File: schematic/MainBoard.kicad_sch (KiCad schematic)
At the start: 0 parts

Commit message: Progress on KiCAD schematics
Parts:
- added U1: LPC1115FBD48-303, Package_QFP:LQFP-48_7x7mm_P0.5mm, symbol MCU_NXP_LPC:LPC1115FBD48-303
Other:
- title: (none) -> Da Vinci Jr. 1.0 Main Board schematic
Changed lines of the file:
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@@
 	(generator_version "10.0")
 	(paper "A4")
+	(title_block
+		(title "Da Vinci Jr. 1.0 Main Board schematic")
+		(date "2026-08-26")
+		(rev "1")
+	)
+	(symbol
+		(lib_id "MCU_NXP_LPC:LPC1115FBD48-303")
+		(at 224.79 73.66 0)
+		(unit 1)
+		(body_style 1)
+		(exclude_from_sim no)
+		(in_bom yes)
+		(on_board yes)
+		(in_pos_files yes)
+		(dnp no)
+		(fields_autoplaced yes)
+		(property "Reference" "U1"
+			(at 229.4733 34.29 0)
+			(show_name no)
+			(do_not_autoplace no)
+			(effects
+				(font
+					(size 1.27 1.27)
+				)
+				(justify left)
+			)
+		)
+		(property "Value" "LPC1115FBD48-303"
+			(at 229.4733 36.83 0)
+			(show_name no)
+			(do_not_autoplace no)
+			(effects
+				(font
+					(size 1.27 1.27)
+				)
+				(justify left)
+			)
+		)
+		(property "Footprint" "Package_QFP:LQFP-48_7x7mm_P0.5mm"
+			(at 247.65 35.56 0)
+			(hide yes)
+			(show_name no)
+			(do_not_autoplace no)
+			(effects
+				(font
+					(size 1.27 1.27)
+				)
+			)
+		)
+		(property "Datasheet" "http://www.nxp.com/docs/en/data-sheet/LPC111X.pdf"
+			(at 273.05 58.42 0)
+			(hide yes)
+			(show_name no)
+			(do_not_autoplace no)
+			(effects
+				(font
+					(size 1.27 1.27)
+				)
+			)
+		)
+		(property "Description" "32-bit ARM Cortex-M0 microcontroller, 64KB flash, 8KB SRAM, power profile"
+			(at 224.79 73.66 0)
+			(hide yes)
+			(show_name no)
+			(do_not_autoplace no)
+			(effects
+				(font
+					(size 1.27 1.27)
+				)
+			)
+		)
+		(pin "14"
+		)
+		(pin "8"
+		)
+		(pin "7"
+		)
+		(pin "9"
+		)
+		(pin "6"
+		)
+		(pin "5"
+		)
+		(pin "13"
+		)
+		(pin "4"
+		)
+		(pin "12"
+		)
+		(pin "11"
+		)
+		(pin "10"
+		)
+		(pin "3"
+		)
+		(pin "17"
+		)
+		(pin "16"
+		)
+		(pin "24"
+		)
+		(pin "25"
+		)
+		(pin "15"
+		)
+		(pin "20"
+		)
+		(pin "26"
+		)
+		(pin "19"
+		)
+		(pin "22"
+		)
+		(pin "18"
+		)
+		(pin "23"
+		)
+		(pin "21"
+		)
+		(pin "2"
+		)
+		(pin "36"
+		)
+		(pin "35"
+		)
+		(pin "34"
+		)
+		(pin "33"
+		)
+		(pin "32"
+		)
+		(pin "31"
+		)
+		(pin "30"
+		)
+		(pin "29"
+		)
+		(pin "28"
+		)
+		(pin "27"
+		)
+		(pin "47"
+		)
+		(pin "46"
+		)
+		(pin "45"
+		)
+		(pin "44"
+		)
+		(pin "43"
+		)
+		(pin "42"
+		)
+		(pin "41"
+		)
+		(pin "48"
+		)
+		(pin "40"
+		)
+		(pin "38"
+		)
+		(pin "39"
+		)
+		(pin "37"
+		)
+		(pin "1"
+		)
+		(instances
+			(project "DaVinciJr1.0"
+				(path "/1e12c736-bef9-40e8-b505-1000ff77a2bb/d610c2e8-63cd-4e0f-98e2-bf1a99df609b"
+					(reference "U1")
+					(unit 1)
+				)
+			)
+		)
+	)
 )

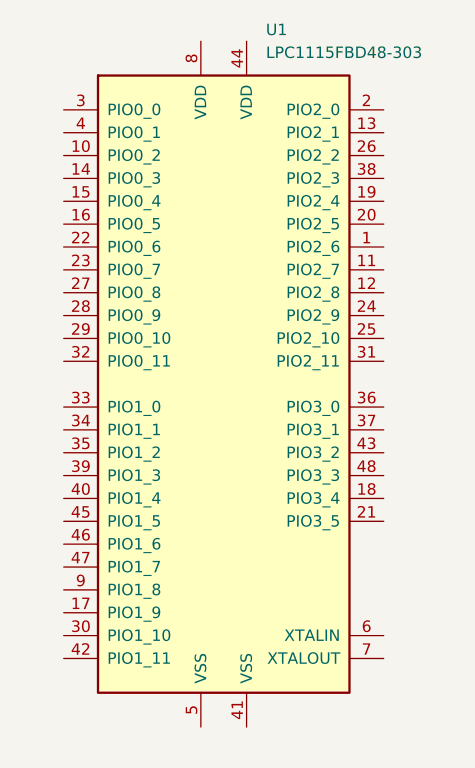
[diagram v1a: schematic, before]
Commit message: Update board schematics
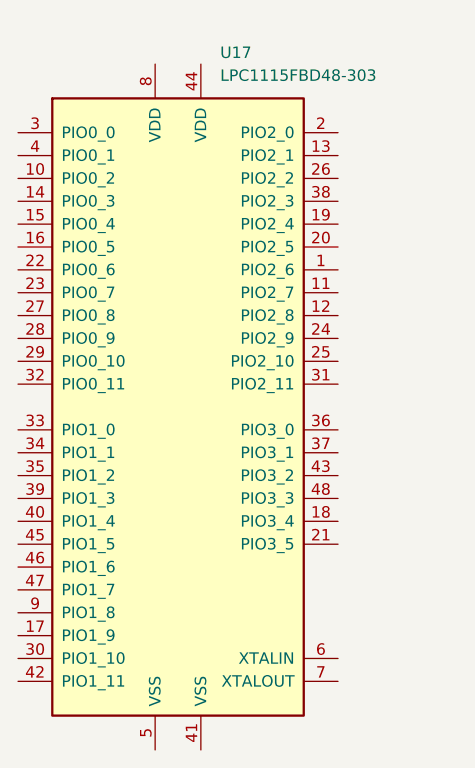
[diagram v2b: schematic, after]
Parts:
- renumbered U1 to U17
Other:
- moved on the sheet: U17
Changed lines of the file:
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@@
 	(symbol
 		(lib_id "MCU_NXP_LPC:LPC1115FBD48-303")
-		(at 224.79 73.66 0)
+		(at 219.71 76.2 0)
 		(unit 1)
 		(body_style 1)
@@
 		(dnp no)
 		(fields_autoplaced yes)
-		(property "Reference" "U1"
-			(at 229.4733 34.29 0)
+		(property "Reference" "U17"
+			(at 224.3933 36.83 0)
 			(show_name no)
 			(do_not_autoplace no)
@@
 		)
 		(property "Value" "LPC1115FBD48-303"
-			(at 229.4733 36.83 0)
+			(at 224.3933 39.37 0)
 			(show_name no)
 			(do_not_autoplace no)
@@
 		)
 		(property "Footprint" "Package_QFP:LQFP-48_7x7mm_P0.5mm"
-			(at 247.65 35.56 0)
+			(at 242.57 38.1 0)
 			(hide yes)
 			(show_name no)
@@
 		)
 		(property "Datasheet" "http://www.nxp.com/docs/en/data-sheet/LPC111X.pdf"
-			(at 273.05 58.42 0)
+			(at 267.97 60.96 0)
 			(hide yes)
 			(show_name no)
@@
 		)
 		(property "Description" "32-bit ARM Cortex-M0 microcontroller, 64KB flash, 8KB SRAM, power profile"
-			(at 224.79 73.66 0)
+			(at 219.71 76.2 0)
 			(hide yes)
 			(show_name no)
@@
 			(project "DaVinciJr1.0"
 				(path "/1e12c736-bef9-40e8-b505-1000ff77a2bb/d610c2e8-63cd-4e0f-98e2-bf1a99df609b"
-					(reference "U1")
+					(reference "U17")
 					(unit 1)
 				)

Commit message: Start main board schematic and update hotend schematic size
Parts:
- added J1, J12, J13, J4, J5: Conn_01x04_Pin, symbol Connector:Conn_01x04_Pin
- added J11: Conn_02x06_Row_Letter_First, symbol Connector_Generic:Conn_02x06_Row_Letter_First
- added J14: Conn_01x03_Pin, symbol Connector:Conn_01x03_Pin
- added J15: Conn_01x02_Pin, symbol Connector:Conn_01x02_Pin
- added J16: Conn_01x06_Pin, symbol Connector:Conn_01x06_Pin
- added J17: USB_B, symbol Connector:USB_B
- added J18: Jack-DC, symbol Connector:Jack-DC
- added SW7: SW_DPST_x2, symbol Switch:SW_DPST_x2
- added U2: ATSAM4E8EA-AU, LQFP144_ATM, symbol 2026-08-26_20-46-55:ATSAM4E8EA-AU
- added U3: MX25L3206E, Package_SO:SOIC-8_5.3x5.3mm_P1.27mm, symbol Memory_Flash:MX25L3233FM2
- added U4, U6, U7, U8: TB62269FTG, Package_QFP:LQFP-48_7x7mm_P0.5mm, symbol TB62269FTG:TB62269FTG
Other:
- moved on the sheet: U17
